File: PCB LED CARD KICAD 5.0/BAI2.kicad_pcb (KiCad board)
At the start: 2 copper layers, 199 x 67 mm, 66 parts, among them J1 Conn_01x08, J10 Conn_01x04, J11 Conn_01x04, J12 Conn_01x04, J13 Conn_01x04, J14 Conn_01x04, J15 Conn_01x04, J16 Conn_01x04, J17 Conn_01x08, J18 Conn_01x04, J19 Conn_01x04, J2 Conn_01x06, J20 Conn_01x04, J21 Conn_01x04, J22 Conn_01x04, J23 Conn_01x04, J24 Conn_01x04, J25 Conn_01x04, J26 Conn_01x06, J27 Conn_01x06, J28 Conn_01x06, J29 Conn_01x06, J3 Conn_01x08, J30 Conn_01x06, J31 Conn_01x08, J32 Conn_01x06, J33 Conn_01x08, J34 Conn_01x06, J35 Conn_01x08, J36 Conn_01x06, J37 Conn_01x08, J38 Conn_01x06, J4 Conn_01x06, J5 Conn_01x08, J6 Conn_01x06, J7 Conn_01x08, J8 Conn_01x06, J9 Conn_01x04, U1 MAX7219, U2 MAX7219, U3 MAX7219, U4 MAX7219

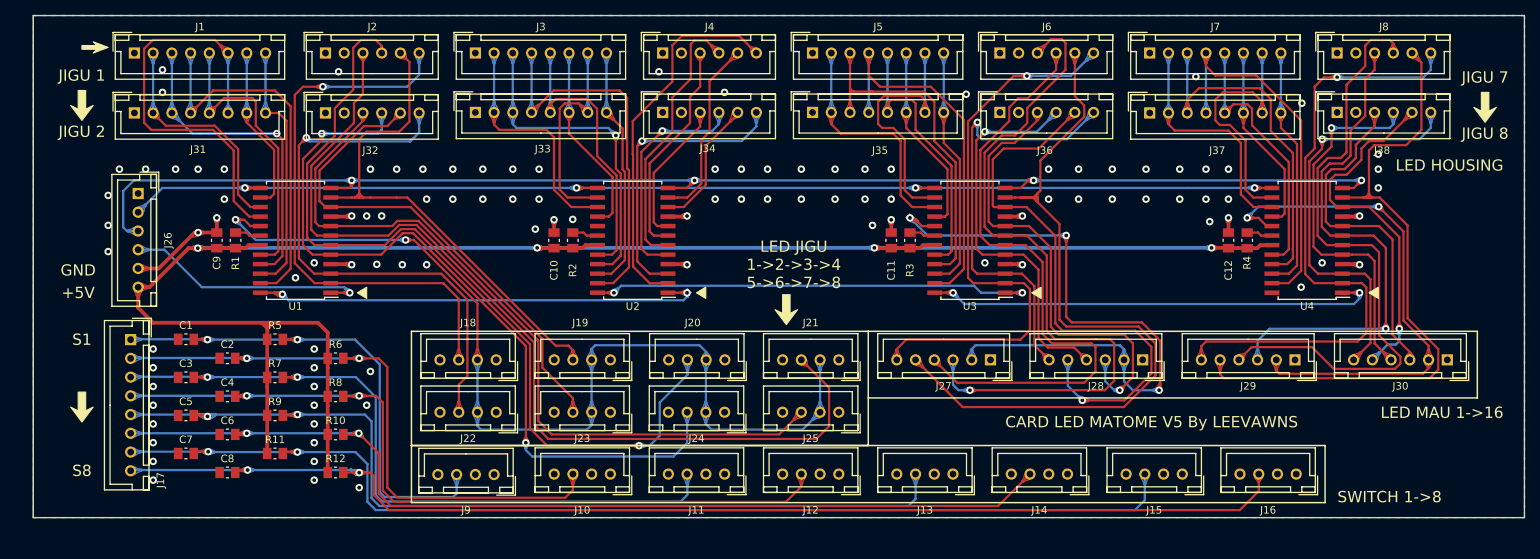
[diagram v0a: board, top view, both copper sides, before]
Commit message: update
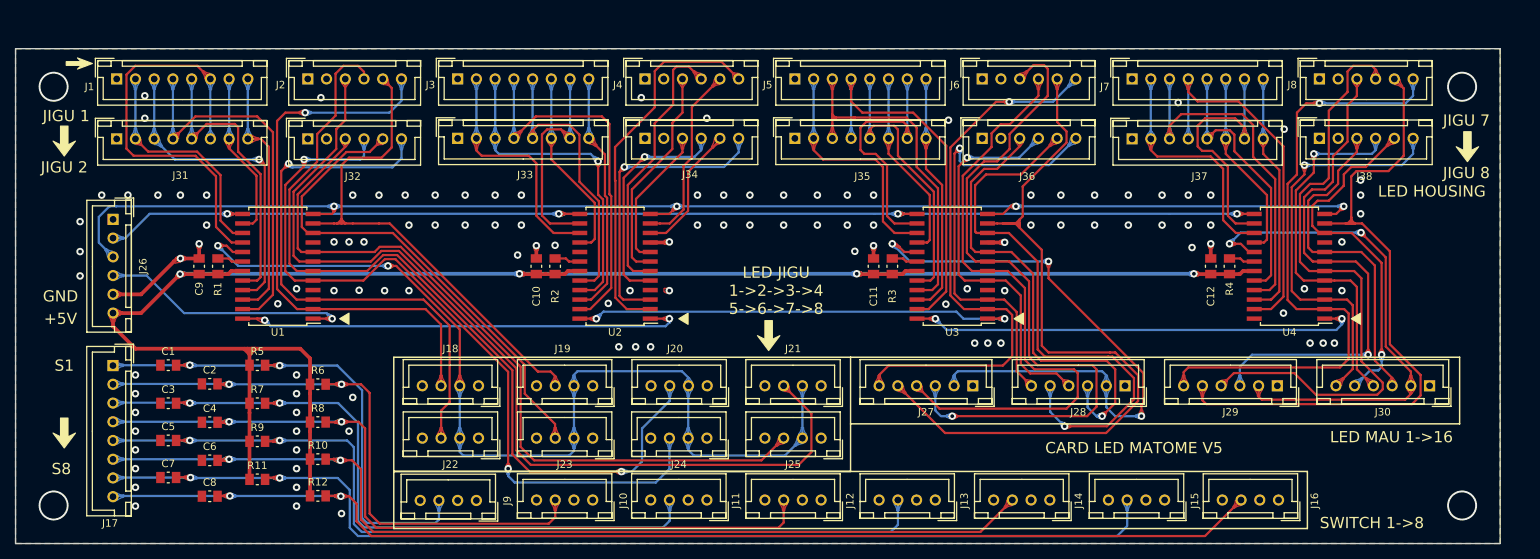
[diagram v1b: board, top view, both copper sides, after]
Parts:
- moved J26 4.81 mm to (53.6, 81.2)
- moved J11 4.19 mm to (132.9, 118.6)
- moved J12 4.19 mm to (148.1, 118.6)
- moved J15 4.19 mm to (194.0, 118.6)
- moved J16 4.19 mm to (209.2, 118.6)
- moved J21 4.19 mm to (148.1, 103.4)
- moved J24 4.19 mm to (132.9, 110.4)
- moved J25 4.19 mm to (148.1, 110.4)
- moved J28 4.19 mm to (188.7, 103.4)
- moved J29 4.19 mm to (209.0, 103.4)
- moved J5 4.19 mm to (144.6, 62.5)
- moved J6 4.19 mm to (169.6, 62.5)
- moved J7 4.19 mm to (189.6, 62.5)
- moved J8 4.19 mm to (214.6, 62.5)
- moved C1 4.19 mm to (61.0, 100.7)
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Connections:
- net VDD renamed +5V
- J1 pad 1: Net-(J1-Pad1) -> (no net)
- J10 pad 1: Net-(J10-Pad1) -> (no net)
- J10 pad 2: Net-(J10-Pad2) -> (no net)
- J11 pad 1: Net-(J11-Pad1) -> (no net)
- J11 pad 2: Net-(J11-Pad2) -> (no net)
- J12 pad 1: Net-(J12-Pad1) -> (no net)
- J12 pad 2: Net-(J12-Pad2) -> (no net)
- J13 pad 1: Net-(J13-Pad1) -> (no net)
- J13 pad 2: Net-(J13-Pad2) -> (no net)
- J14 pad 1: Net-(J14-Pad1) -> (no net)
- J14 pad 2: Net-(J14-Pad2) -> (no net)
- J15 pad 1: Net-(J15-Pad1) -> (no net)
- J15 pad 2: Net-(J15-Pad2) -> (no net)
- J16 pad 1: Net-(J16-Pad1) -> (no net)
- J16 pad 2: Net-(J16-Pad2) -> (no net)
- J18 pad 1: Net-(J18-Pad1) -> (no net)
- J18 pad 4: Net-(J18-Pad4) -> (no net)
- J19 pad 1: Net-(J19-Pad1) -> (no net)
- J19 pad 4: Net-(J19-Pad4) -> (no net)
- J2 pad 1: Net-(J2-Pad1) -> (no net)
- J2 pad 2: Net-(J2-Pad2) -> (no net)
- J20 pad 1: Net-(J20-Pad1) -> (no net)
- J20 pad 4: Net-(J20-Pad4) -> (no net)
- J21 pad 1: Net-(J21-Pad1) -> (no net)
- J21 pad 4: Net-(J21-Pad4) -> (no net)
- J22 pad 1: Net-(J22-Pad1) -> (no net)
- J22 pad 4: Net-(J22-Pad4) -> (no net)
- J23 pad 1: Net-(J23-Pad1) -> (no net)
- J23 pad 4: Net-(J23-Pad4) -> (no net)
- J24 pad 1: Net-(J24-Pad1) -> (no net)
- J24 pad 4: Net-(J24-Pad4) -> (no net)
- J25 pad 1: Net-(J25-Pad1) -> (no net)
- J25 pad 4: Net-(J25-Pad4) -> (no net)
- J26 pad 1: Net-(J26-Pad1) -> (no net)
- J27 pad 1: Net-(J27-Pad1) -> (no net)
- J28 pad 1: Net-(J28-Pad1) -> (no net)
- J29 pad 1: Net-(J29-Pad1) -> (no net)
- J3 pad 1: Net-(J3-Pad1) -> (no net)
- J30 pad 1: Net-(J30-Pad1) -> (no net)
- J31 pad 1: Net-(J31-Pad1) -> (no net)
- J32 pad 1: Net-(J32-Pad1) -> (no net)
- J32 pad 2: Net-(J32-Pad2) -> (no net)
- J33 pad 1: Net-(J33-Pad1) -> (no net)
- J34 pad 1: Net-(J34-Pad1) -> (no net)
- J34 pad 2: Net-(J34-Pad2) -> (no net)
- J35 pad 1: Net-(J35-Pad1) -> (no net)
- J36 pad 1: Net-(J36-Pad1) -> (no net)
- J36 pad 2: Net-(J36-Pad2) -> (no net)
- J37 pad 1: Net-(J37-Pad1) -> (no net)
- J38 pad 1: Net-(J38-Pad1) -> (no net)
- J38 pad 2: Net-(J38-Pad2) -> (no net)
- J4 pad 1: Net-(J4-Pad1) -> (no net)
- J4 pad 2: Net-(J4-Pad2) -> (no net)
- J5 pad 1: Net-(J5-Pad1) -> (no net)
- J6 pad 1: Net-(J6-Pad1) -> (no net)
- J6 pad 2: Net-(J6-Pad2) -> (no net)
- J7 pad 1: Net-(J7-Pad1) -> (no net)
- J8 pad 1: Net-(J8-Pad1) -> (no net)
- J8 pad 2: Net-(J8-Pad2) -> (no net)
- J9 pad 1: Net-(J9-Pad1) -> (no net)
- J9 pad 2: Net-(J9-Pad2) -> (no net)
- U2 pad 17: Net-(U2-Pad17) -> (no net)
- U4 pad 24: Net-(U4-Pad24) -> (no net)
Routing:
- net VSS: track 40.0 -> 26.3 mm, vias 106 -> 119
- net /3-C8: track 88.6 -> 83.2 mm
- net +5V: track 248.0 -> 249.8 mm
- net /SW8: track 161.5 -> 160.1 mm
- net /DIN: track 33.2 -> 34.2 mm
- net /CLK: track 160.1 -> 161.1 mm
- net /SW4: track 108.5 -> 109.3 mm
- net /SW6: track 132.7 -> 133.5 mm
- net /2-R5: track 39.0 -> 39.7 mm
- net /3-R1: track 76.0 -> 75.4 mm
- net (no net): vias 0 -> 3
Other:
- board size 199 x 67 mm -> 198.1 x 66 mm
- board text added: "CARD LED MATOME V5"
- board text removed: "CARD LED MATOME V5 By LEEVAWNS"
